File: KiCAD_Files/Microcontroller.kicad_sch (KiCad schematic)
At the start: 22 parts, among them U901 OwnTech_SPIN, U902 WE-TVS-824015043, U903 WE-TVS-824015043

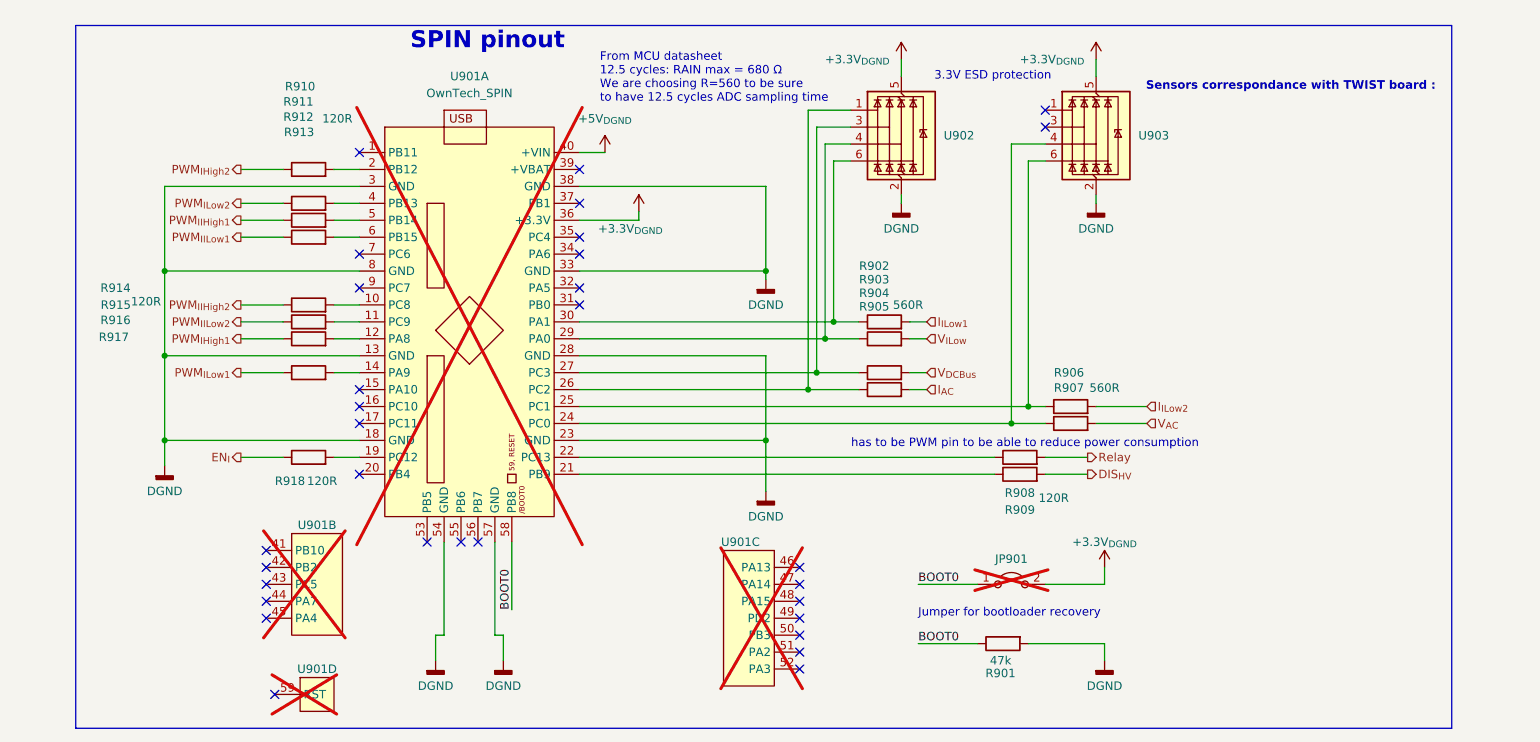
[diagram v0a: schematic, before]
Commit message: Tidied up the schematic. Added the pdf version for V0.9.
Signed-off-by: Jean Alinei <jean.alinei@owntech.org>
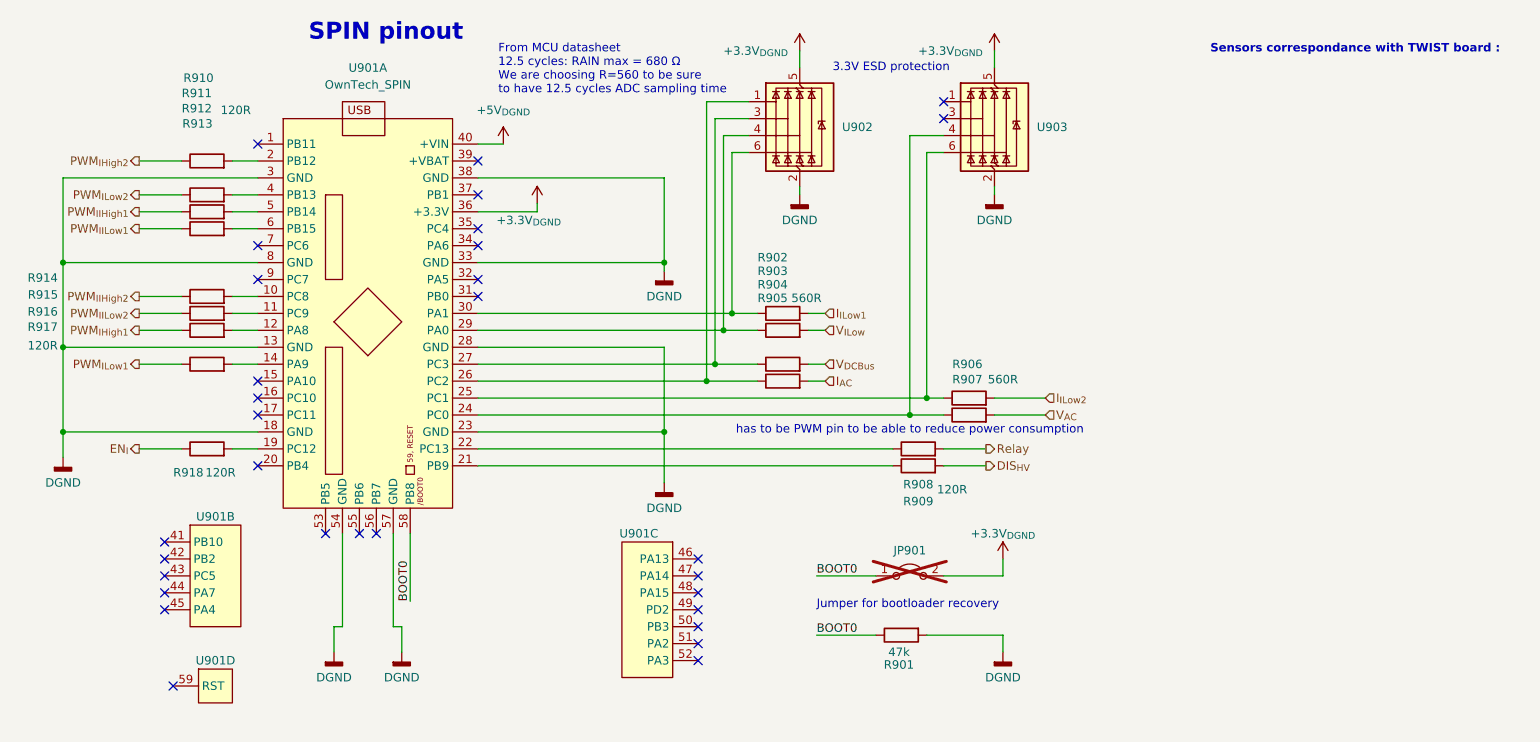
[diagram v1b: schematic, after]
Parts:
- U901: now fitted
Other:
- title: Micro-inverter - 400W -> Power stage controller
- moved on the sheet: JP901, R901, R902, R903, R904, R905, R906, R907, R908, R909, R910, R911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
